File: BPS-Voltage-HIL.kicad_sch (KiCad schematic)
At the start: 3 parts, among them J3 SOMConnector, U2 DAC7311xDCK, U4 DAC7311xDCK

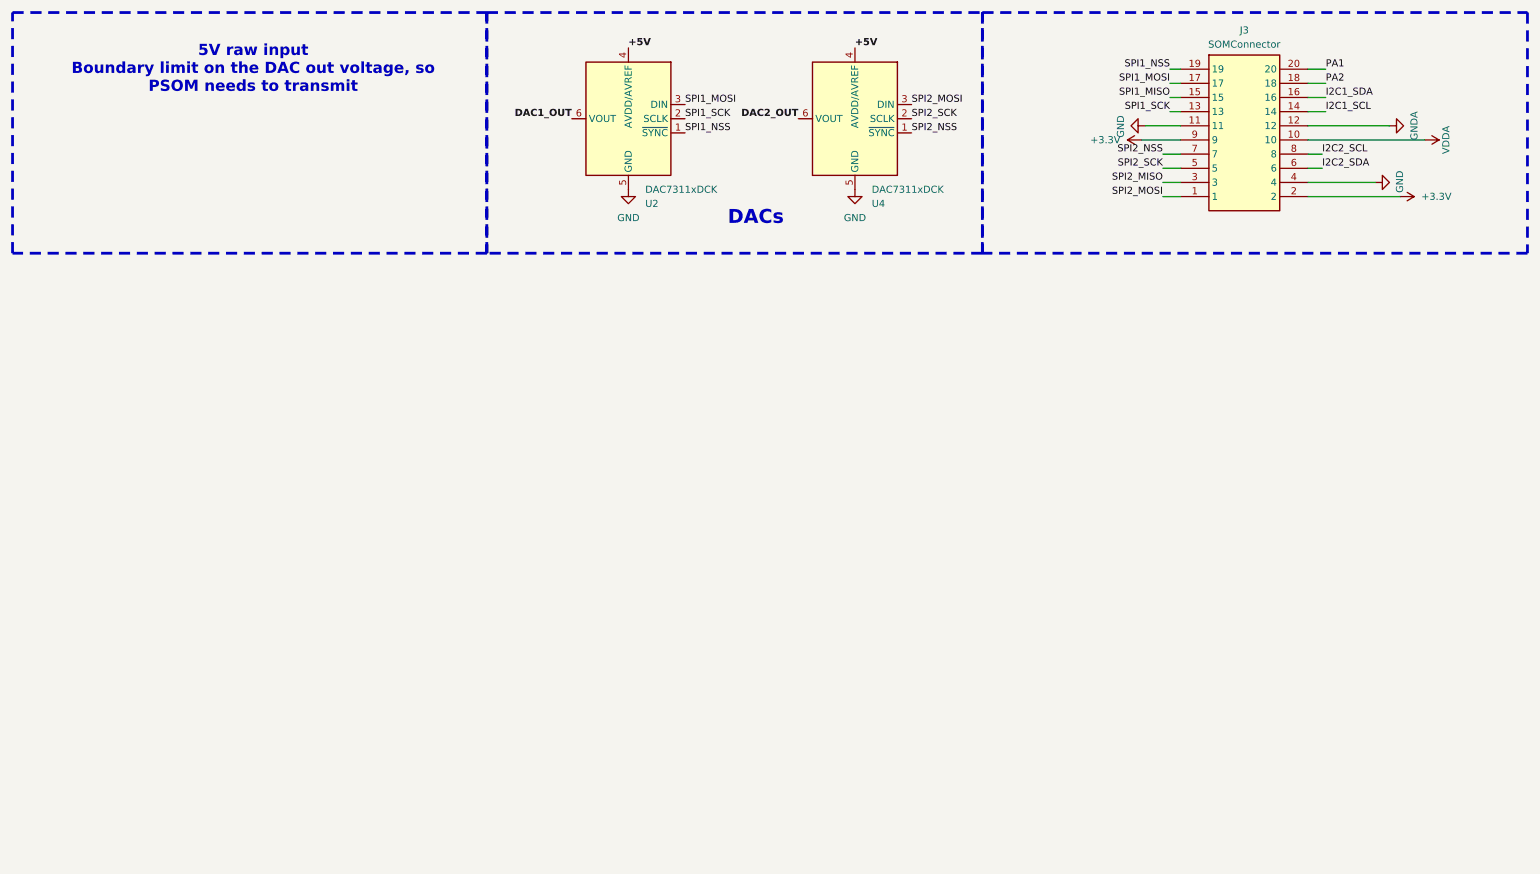
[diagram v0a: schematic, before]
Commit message: push
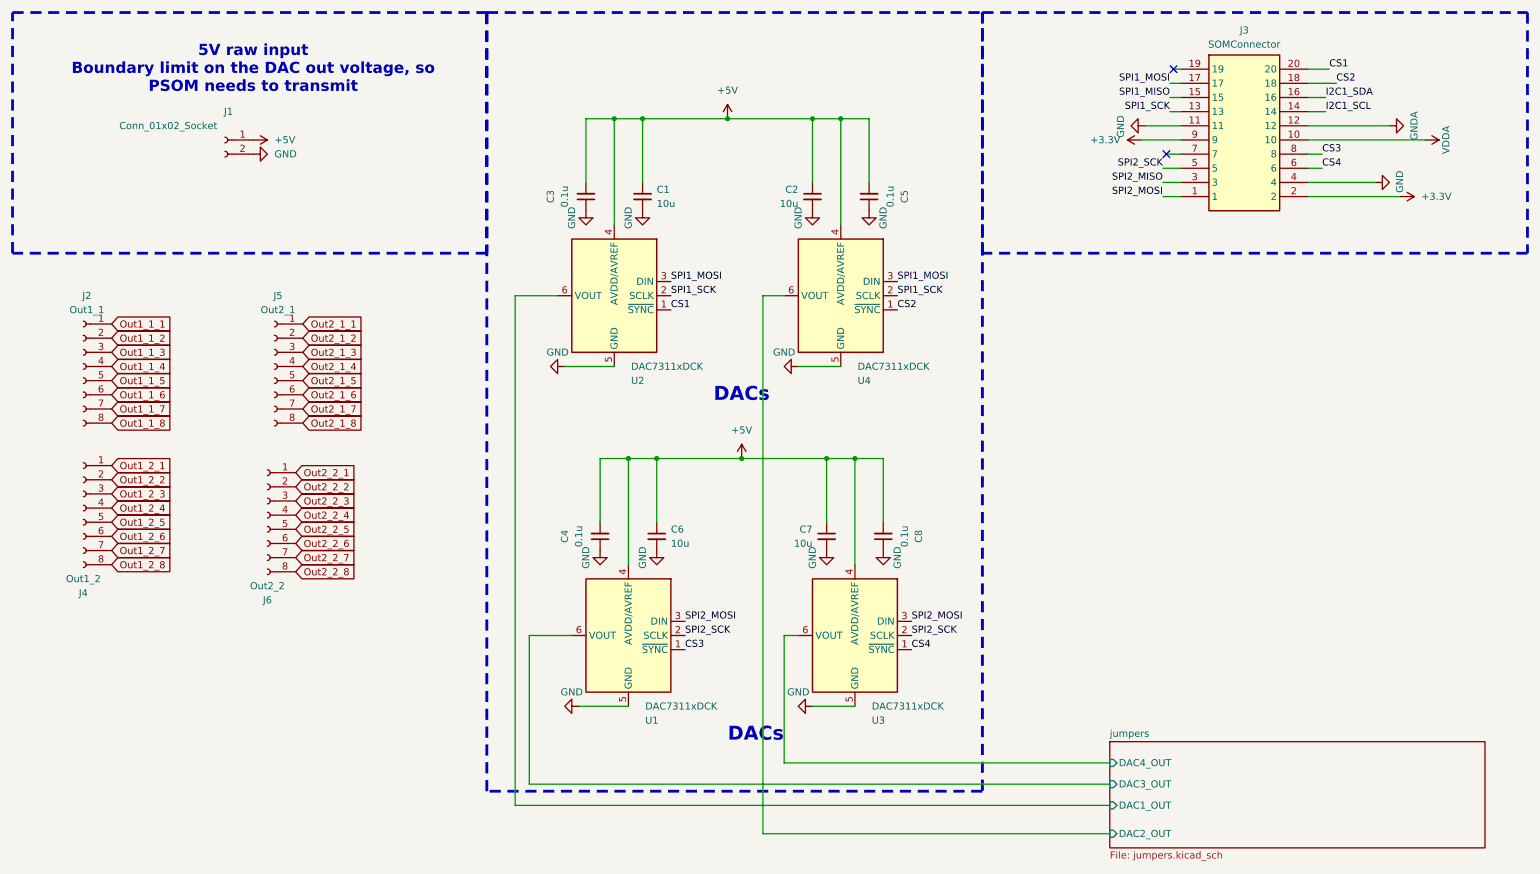
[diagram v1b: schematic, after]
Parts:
- added C1, C2, C6, C7: 10u, Capacitor_SMD:C_0805_2012Metric_Pad1.18x1.45mm_HandSolder, symbol Device:C_Small
- added C3, C4, C5, C8: 0.1u, Capacitor_SMD:C_0805_2012Metric_Pad1.18x1.45mm_HandSolder, symbol Device:C_Small
- added J1: Conn_01x02_Socket, Connector_Molex:Molex_Micro-Fit_3.0_43045-0212_2x01_P3.00mm_Vertical, symbol Connector:Conn_01x02_Socket
- added J2: Out1_1, Connector_Molex:Molex_Micro-Fit_3.0_43650-0815_1x08_P3.00mm_Vertical, symbol Connector:Conn_01x08_Socket
- added J4: Out1_2, Connector_Molex:Molex_Micro-Fit_3.0_43650-0815_1x08_P3.00mm_Vertical, symbol Connector:Conn_01x08_Socket
- added J5: Out2_1, Connector_Molex:Molex_Micro-Fit_3.0_43650-0815_1x08_P3.00mm_Vertical, symbol Connector:Conn_01x08_Socket
- added J6: Out2_2, Connector_Molex:Molex_Micro-Fit_3.0_43650-0815_1x08_P3.00mm_Vertical, symbol Connector:Conn_01x08_Socket
- added U1, U3: DAC7311xDCK, Package_TO_SOT_SMD:SOT-363_SC-70-6, symbol Analog_DAC:DAC7311xDCK
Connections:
- net +5V: now also C1.1, C2.1, C3.2, C4.2, C5.2, C6.1, C7.1, C8.2, J1.1 (Pin_1), U1.4 (AVDD/AVREF), U3.4 (AVDD/AVREF)
- net GND: now also C1.2, C2.2, C3.1, C4.1, C5.1, C6.2, C7.2, C8.1, J1.2 (Pin_2), U1.5 (GND), U3.5 (GND)
- net SPI1_MOSI: now also U4.3 (DIN)
- net SPI1_SCK: now also U4.2 (SCLK)
- net SPI2_MOSI: now also U1.3 (DIN), U3.3 (DIN); no longer U4.3 (DIN)
- net SPI2_SCK: now also U1.2 (SCLK), U3.2 (SCLK); no longer U4.2 (SCLK)
- net DAC1_OUT renamed jumpers/DAC1_OUT
- net DAC2_OUT renamed jumpers/DAC2_OUT
- net I2C2_SCL renamed CS3
- net CS3: now also U1.1 (~{SYNC})
- net I2C2_SDA renamed CS4
- net CS4: now also U3.1 (~{SYNC})
- net PA1 renamed CS1
- net CS1: now also U2.1 (~{SYNC})
- net PA2 renamed CS2
- net CS2: now also U4.1 (~{SYNC})
- net SPI1_NSS: no longer names the net of J3.19
- net SPI1_NSS: no longer U2.1 (~{SYNC})
- net SPI2_NSS: no longer names the net of J3.7
- net SPI2_NSS: no longer U4.1 (~{SYNC})
- new net Out1_1_1: J2.1 (Pin_1)
- new net Out1_1_2: J2.2 (Pin_2)
- new net Out1_1_3: J2.3 (Pin_3)
- new net Out1_1_4: J2.4 (Pin_4)
- new net Out1_1_5: J2.5 (Pin_5)
- new net Out1_1_6: J2.6 (Pin_6)
- new net Out1_1_7: J2.7 (Pin_7)
- new net Out1_1_8: J2.8 (Pin_8)
- new net Out1_2_1: J4.1 (Pin_1)
- new net Out1_2_2: J4.2 (Pin_2)
- new net Out1_2_3: J4.3 (Pin_3)
- new net Out1_2_4: J4.4 (Pin_4)
- new net Out1_2_5: J4.5 (Pin_5)
- new net Out1_2_6: J4.6 (Pin_6)
- new net Out1_2_7: J4.7 (Pin_7)
- new net Out1_2_8: J4.8 (Pin_8)
- new net Out2_1_1: J5.1 (Pin_1)
- new net Out2_1_2: J5.2 (Pin_2)
- new net Out2_1_3: J5.3 (Pin_3)
- new net Out2_1_4: J5.4 (Pin_4)
- new net Out2_1_5: J5.5 (Pin_5)
- new net Out2_1_6: J5.6 (Pin_6)
- new net Out2_1_7: J5.7 (Pin_7)
- new net Out2_1_8: J5.8 (Pin_8)
- new net Out2_2_1: J6.1 (Pin_1)
- new net Out2_2_2: J6.2 (Pin_2)
- new net Out2_2_3: J6.3 (Pin_3)
- new net Out2_2_4: J6.4 (Pin_4)
- new net Out2_2_5: J6.5 (Pin_5)
- new net Out2_2_6: J6.6 (Pin_6)
- new net Out2_2_7: J6.7 (Pin_7)
- new net Out2_2_8: J6.8 (Pin_8)
- new net jumpers/DAC3_OUT: U1.6 (VOUT)
- new net jumpers/DAC4_OUT: U3.6 (VOUT)
- no-connect marks 0 -> 2
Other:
- added sheet jumpers (jumpers.kicad_sch)
- moved on the sheet: U2, U4
